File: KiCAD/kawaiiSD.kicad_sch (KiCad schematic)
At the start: 11 parts, among them J1 503398-1892

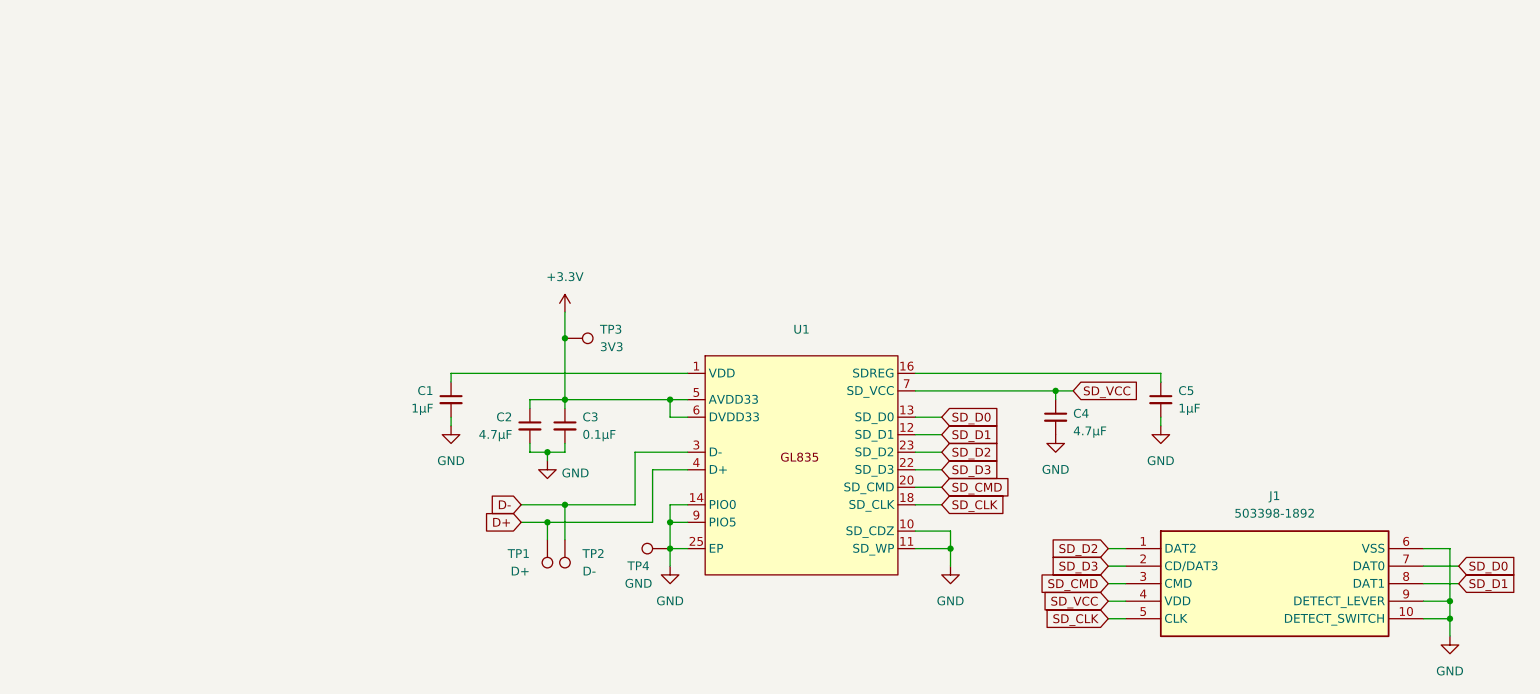
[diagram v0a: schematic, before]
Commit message: initial commit
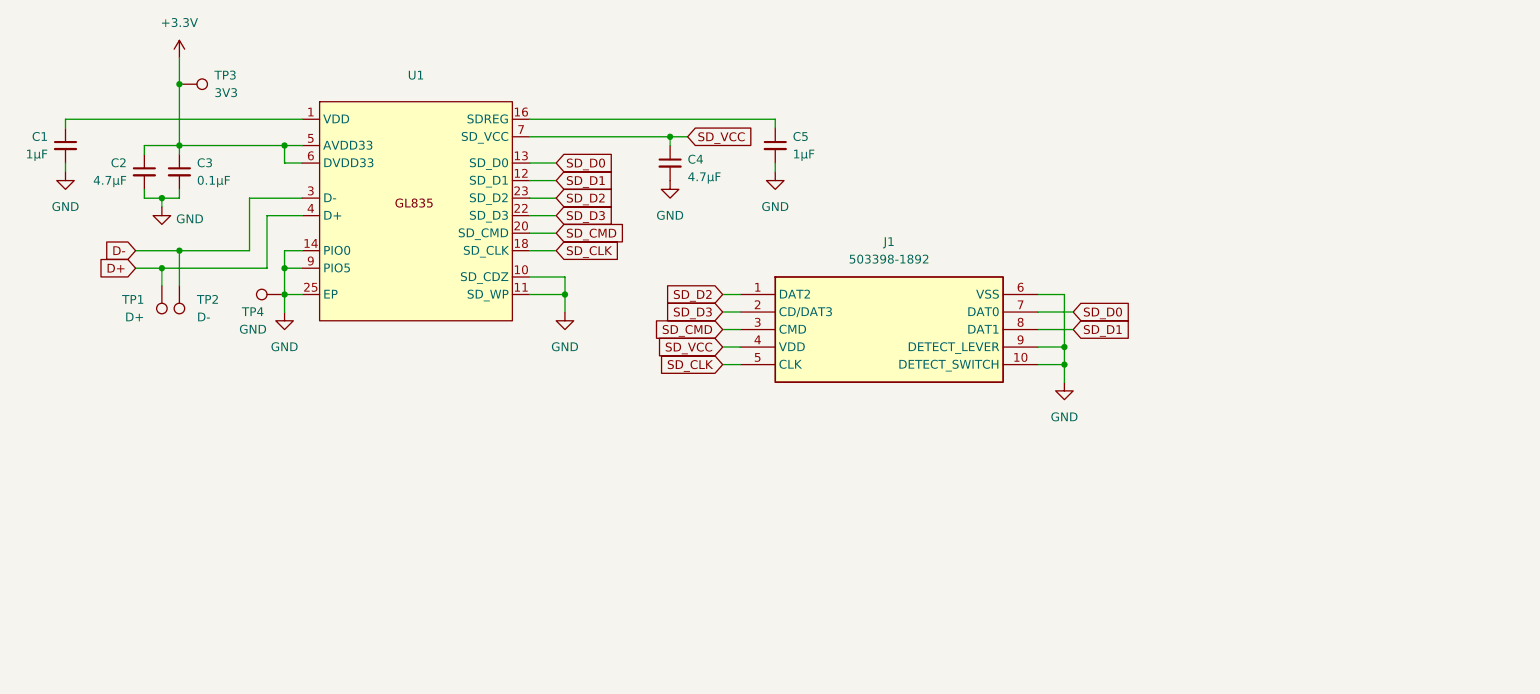
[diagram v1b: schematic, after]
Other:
- moved on the sheet: C1, C2, C3, C4, C5, J1, TP1, TP2, TP3, TP4, U1
